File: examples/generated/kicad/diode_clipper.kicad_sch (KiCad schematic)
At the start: 3 parts

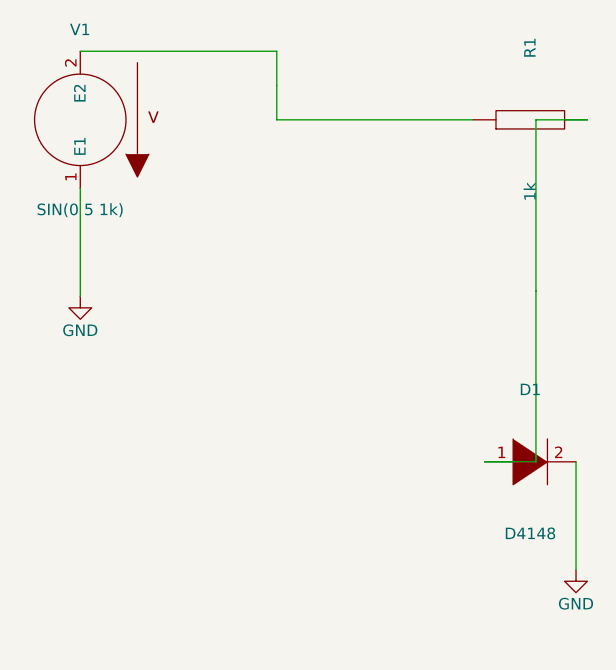
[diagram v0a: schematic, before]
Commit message: Attempt to correct strange wiring.
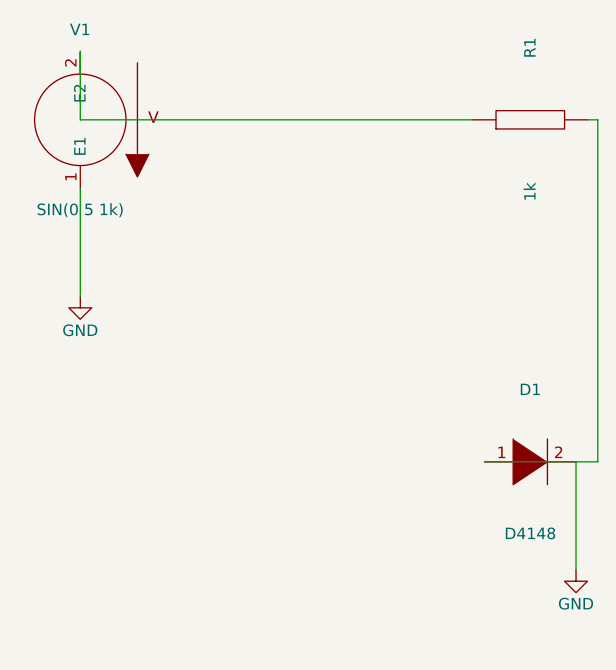
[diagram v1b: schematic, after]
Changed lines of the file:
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@@
     (stroke (width 0) (type solid) (color 0 0 0 0))
   )
-  (wire (pts (xy 50.00 62.38) (xy 71.83 62.38))
+  (wire (pts (xy 50.00 62.38) (xy 50.00 70.00))
     (stroke (width 0) (type solid) (color 0 0 0 0))
   )
-  (wire (pts (xy 71.83 62.38) (xy 71.83 66.19))
+  (wire (pts (xy 50.00 70.00) (xy 93.65 70.00))
     (stroke (width 0) (type solid) (color 0 0 0 0))
   )
-  (wire (pts (xy 93.65 70.00) (xy 71.83 70.00))
+  (wire (pts (xy 106.35 70.00) (xy 107.50 70.00))
     (stroke (width 0) (type solid) (color 0 0 0 0))
   )
-  (wire (pts (xy 71.83 70.00) (xy 71.83 66.19))
+  (wire (pts (xy 107.50 70.00) (xy 107.50 108.00))
     (stroke (width 0) (type solid) (color 0 0 0 0))
   )
-  (wire (pts (xy 106.35 70.00) (xy 100.63 70.00))
+  (wire (pts (xy 107.50 108.00) (xy 94.92 108.00))
     (stroke (width 0) (type solid) (color 0 0 0 0))
   )
-  (wire (pts (xy 100.63 70.00) (xy 100.63 89.00))
-    (stroke (width 0) (type solid) (color 0 0 0 0))
-  )
-  (wire (pts (xy 94.92 108.00) (xy 100.63 108.00))
-    (stroke (width 0) (type solid) (color 0 0 0 0))
-  )
-  (wire (pts (xy 100.63 108.00) (xy 100.63 89.00))
-    (stroke (width 0) (type solid) (color 0 0 0 0))
-  )

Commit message: Attempt shape and wiring fixes again.
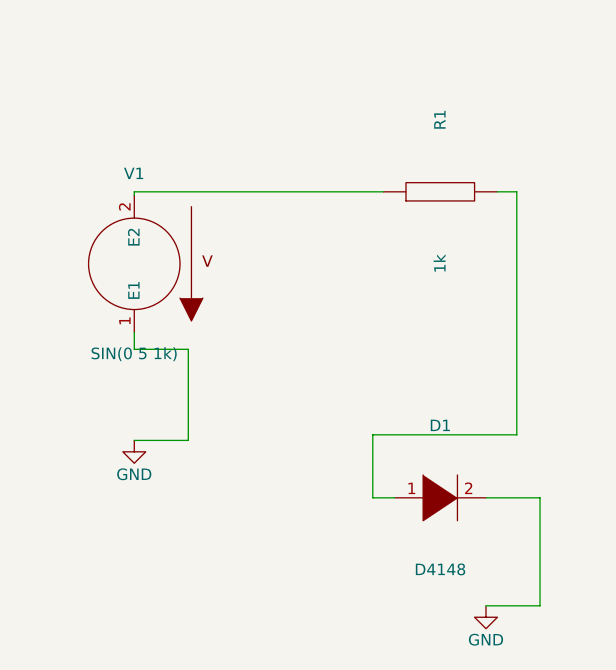
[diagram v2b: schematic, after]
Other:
- moved on the sheet: D1, R1, V1
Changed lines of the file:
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@@
     (comment 1 "Generated by mixedsig2cad")
   )
-  (symbol (lib_id "VSOURCE") (at 50.00 70.00 180) (unit 1)
+  (symbol (lib_id "VSOURCE") (at 56.00 86.00 180) (unit 1)
     (in_bom yes) (on_board yes)
-    (property "Reference" "V1" (at 50.0 60.0 0)
+    (property "Reference" "V1" (at 56.0 76.0 0)
       (effects (font (size 1.27 1.27)))
     )
-    (property "Value" "SIN(0 5 1k)" (at 50.0 80.0 0)
+    (property "Value" "SIN(0 5 1k)" (at 56.0 96.0 0)
       (effects (font (size 1.27 1.27)))
     )
@@
     )
   )
-  (symbol (lib_id "R") (at 100.00 70.00 90) (unit 1)
+  (symbol (lib_id "R") (at 90.00 78.00 90) (unit 1)
     (in_bom yes) (on_board yes)
-    (property "Reference" "R1" (at 100.0 62.0 0)
+    (property "Reference" "R1" (at 90.0 70.0 0)
       (effects (font (size 1.27 1.27)))
     )
-    (property "Value" "1k" (at 100.0 78.0 0)
+    (property "Value" "1k" (at 90.0 86.0 0)
       (effects (font (size 1.27 1.27)))
     )
@@
     )
   )
-  (symbol (lib_id "DIODE") (at 100.00 108.00 0) (unit 1)
+  (symbol (lib_id "DIODE") (at 90.00 112.00 0) (unit 1)
     (in_bom yes) (on_board yes)
-    (property "Reference" "D1" (at 100.0 100.0 0)
+    (property "Reference" "D1" (at 90.0 104.0 0)
       (effects (font (size 1.27 1.27)))
     )
-    (property "Value" "D4148" (at 100.0 116.0 0)
+    (property "Value" "D4148" (at 90.0 120.0 0)
       (effects (font (size 1.27 1.27)))
     )
@@
     )
   )
-  (symbol (lib_id "GND") (at 50.00 89.62 0) (unit 1)
+  (symbol (lib_id "GND") (at 56.00 105.62 0) (unit 1)
     (in_bom yes) (on_board yes)
-    (property "Reference" "#PWR0001" (at 50.0 85.81 0)
+    (property "Reference" "#PWR0001" (at 56.0 101.81 0)
       (effects (font (size 1.27 1.27)) hide)
     )
-    (property "Value" "GND" (at 50.0 93.43 0)
+    (property "Value" "GND" (at 56.0 109.43 0)
       (effects (font (size 1.27 1.27)))
     )
@@
     )
   )
-  (symbol (lib_id "GND") (at 105.08 120.00 0) (unit 1)
+  (symbol (lib_id "GND") (at 95.08 124.00 0) (unit 1)
     (in_bom yes) (on_board yes)
-    (property "Reference" "#PWR0002" (at 105.08 116.19 0)
+    (property "Reference" "#PWR0002" (at 95.08 120.19 0)
       (effects (font (size 1.27 1.27)) hide)
     )
-    (property "Value" "GND" (at 105.08 123.81 0)
+    (property "Value" "GND" (at 95.08 127.81 0)
       (effects (font (size 1.27 1.27)))
     )
@@
     )
   )
-  (wire (pts (xy 50.00 77.62) (xy 50.00 89.62))
+  (wire (pts (xy 56.00 93.62) (xy 56.00 95.50))
     (stroke (width 0) (type solid) (color 0 0 0 0))
   )
-  (wire (pts (xy 105.08 108.00) (xy 105.08 120.00))
+  (wire (pts (xy 56.00 95.50) (xy 62.00 95.50))
     (stroke (width 0) (type solid) (color 0 0 0 0))
   )
-  (wire (pts (xy 50.00 62.38) (xy 50.00 70.00))
+  (wire (pts (xy 62.00 95.50) (xy 62.00 105.62))
     (stroke (width 0) (type solid) (color 0 0 0 0))
   )
-  (wire (pts (xy 50.00 70.00) (xy 93.65 70.00))
+  (wire (pts (xy 62.00 105.62) (xy 56.00 105.62))
     (stroke (width 0) (type solid) (color 0 0 0 0))
   )
-  (wire (pts (xy 106.35 70.00) (xy 107.50 70.00))
+  (wire (pts (xy 95.08 112.00) (xy 101.08 112.00))
     (stroke (width 0) (type solid) (color 0 0 0 0))
   )
-  (wire (pts (xy 107.50 70.00) (xy 107.50 108.00))
+  (wire (pts (xy 101.08 112.00) (xy 101.08 124.00))
     (stroke (width 0) (type solid) (color 0 0 0 0))
   )
-  (wire (pts (xy 107.50 108.00) (xy 94.92 108.00))
+  (wire (pts (xy 101.08 124.00) (xy 95.08 124.00))
     (stroke (width 0) (type solid) (color 0 0 0 0))
   )
+  (wire (pts (xy 56.00 78.38) (xy 56.00 78.00))
+    (stroke (width 0) (type solid) (color 0 0 0 0))
+  )
+  (wire (pts (xy 56.00 78.00) (xy 83.65 78.00))
+    (stroke (width 0) (type solid) (color 0 0 0 0))
+  )
+  (wire (pts (xy 96.35 78.00) (xy 98.50 78.00))
+    (stroke (width 0) (type solid) (color 0 0 0 0))
+  )
+  (wire (pts (xy 98.50 78.00) (xy 98.50 105.00))
+    (stroke (width 0) (type solid) (color 0 0 0 0))
+  )
+  (wire (pts (xy 98.50 105.00) (xy 82.50 105.00))
+    (stroke (width 0) (type solid) (color 0 0 0 0))
+  )
+  (wire (pts (xy 82.50 105.00) (xy 82.50 112.00))
+    (stroke (width 0) (type solid) (color 0 0 0 0))
+  )
+  (wire (pts (xy 82.50 112.00) (xy 84.92 112.00))
+    (stroke (width 0) (type solid) (color 0 0 0 0))
+  )
